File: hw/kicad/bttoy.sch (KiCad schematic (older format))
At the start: 4 parts

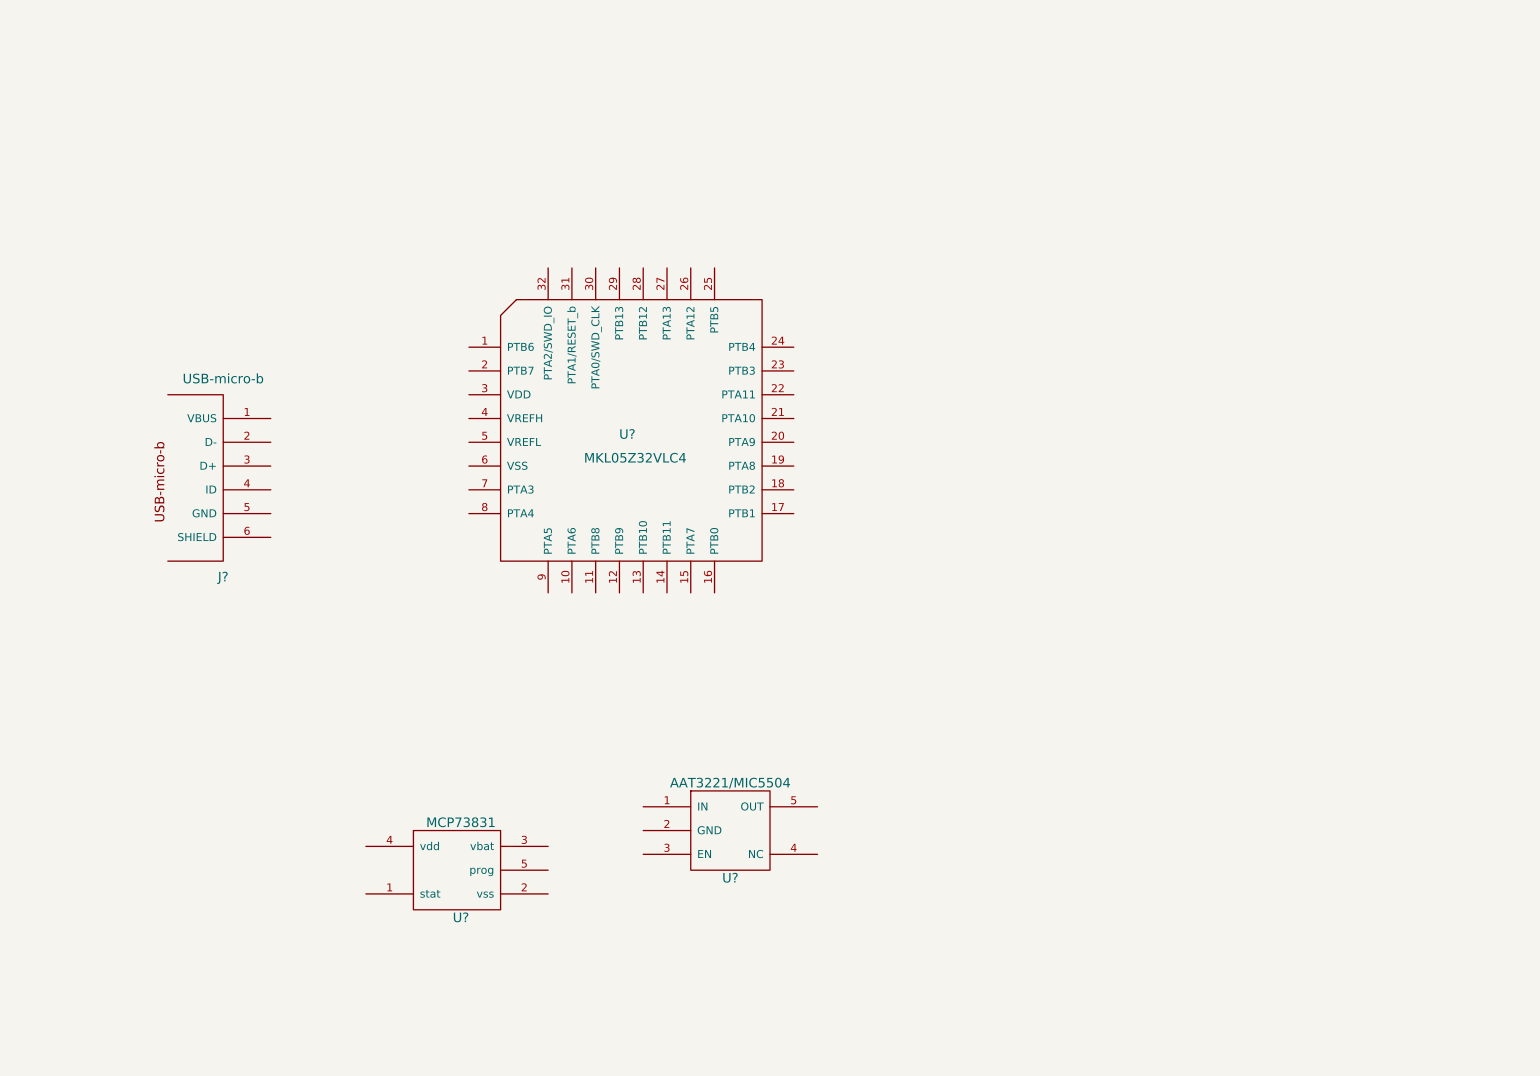
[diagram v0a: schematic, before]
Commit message: - start flushing out subsystems
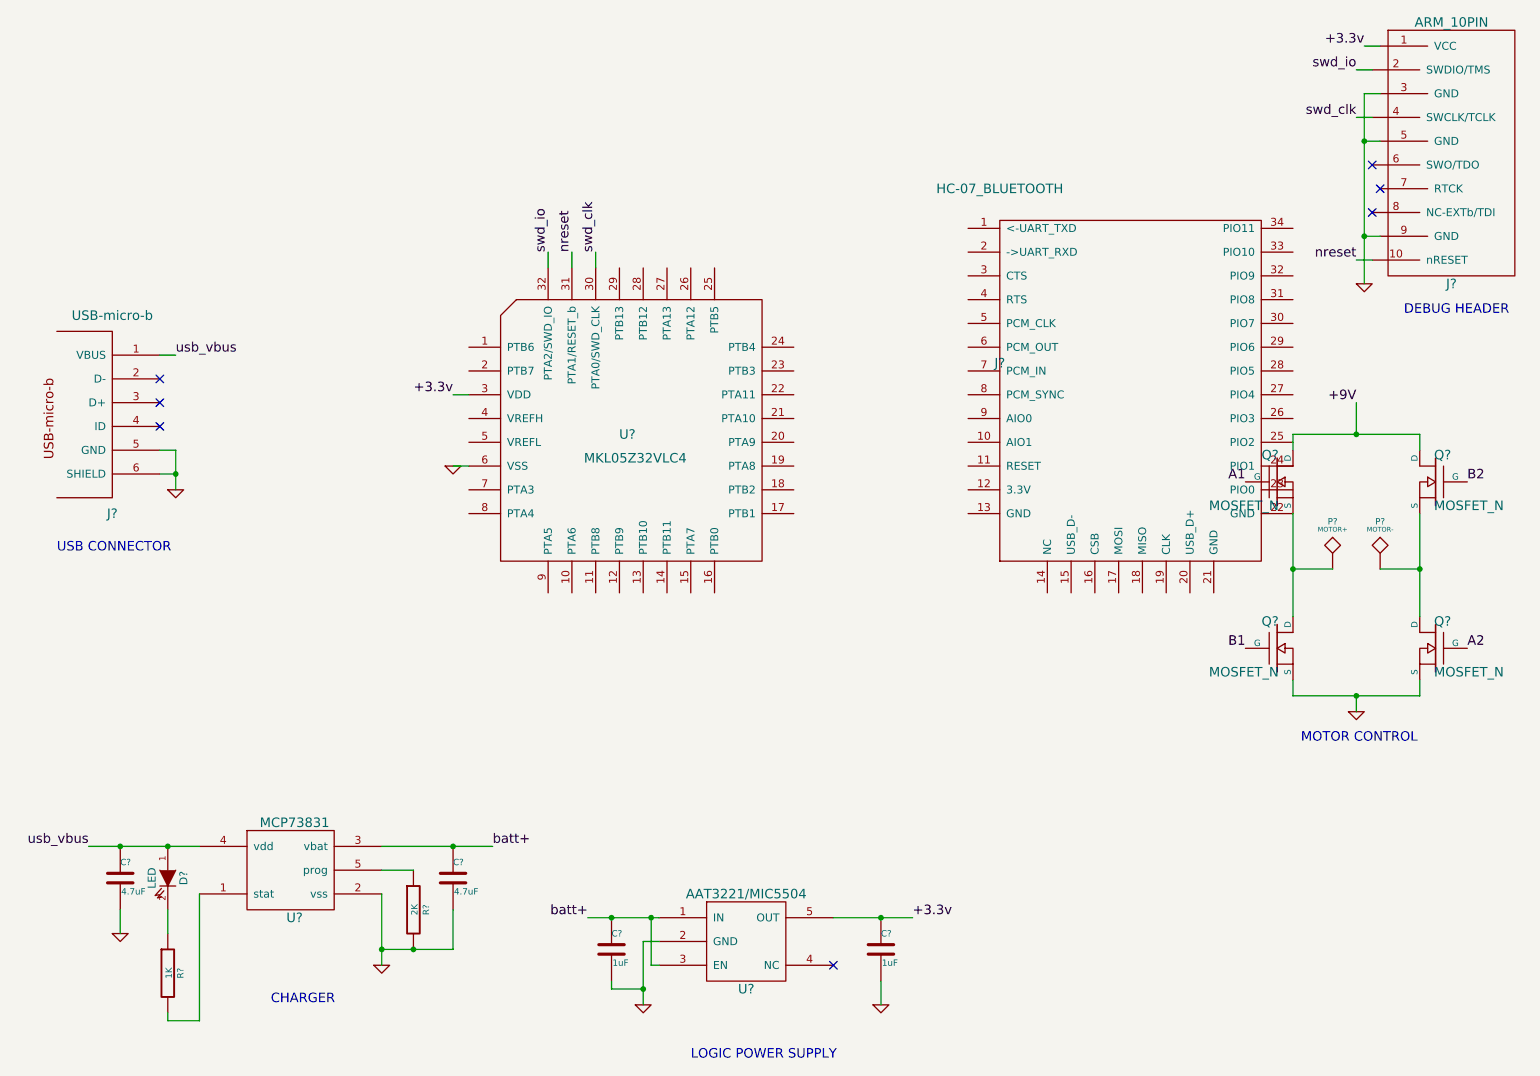
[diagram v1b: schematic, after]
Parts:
- added C? (x2): 4.7uF, symbol C
- added C? (x2): 1uF, symbol C
- added D?: LED, symbol LED
- added J?: ARM_10PIN, symbol ARM_10PIN
- added J?: HC-07_BLUETOOTH, symbol HC-07_BLUETOOTH
- added P?: MOTOR+, symbol TST
- added P?: MOTOR-, symbol TST
- added Q? (x4): MOSFET_N, symbol MOSFET_N
- added R?: 1K, symbol R
- added R?: 2K, symbol R
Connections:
- net +3.3v: now reaches U?.3 (VDD)
- net +3.3v: now also U?.5 (OUT), C?.1, J?.1 (VCC)
- net swd_clk: now reaches U?.30 (PTA0/SWD_CLK)
- net swd_clk: now also J?.4 (SWCLK/TCLK)
- net nreset: now reaches U?.31 (PTA1/RESET_b)
- net nreset: now also J?.10 (nRESET)
- net swd_io: now reaches U?.32 (PTA2/SWD_IO)
- net swd_io: now also J?.2 (SWDIO/TMS)
- net GND: now reaches U?.6 (VSS)
- net GND: now also J?.5 (GND), J?.6 (SHIELD), U?.2 (GND), U?.2 (vss), C?.2, C?.2, C?.2, C?.2, J?.3 (GND), J?.5 (GND), J?.9 (GND), Q?.S, Q?.S, R?.2
- net at U?.1 (stat): now also R?.2
- net batt+: now reaches U?.3 (vbat)
- net batt+: now also U?.1 (IN), U?.3 (EN), C?.1, C?.1
- net usb_vbus: now reaches U?.4 (vdd)
- net usb_vbus: now also J?.1 (VBUS), C?.1, D?.1 (A)
- net at U?.5 (prog): now also R?.1
- new net: J?.22 (GND), P?.1, Q?.D, Q?.S
- new net: P?.1, Q?.D, Q?.S
- new net: D?.2 (K), R?.1
- new net +9V: Q?.D, Q?.D
- new net A1: Q?.G
- new net A2: Q?.G
- new net B1: Q?.G
- new net B2: Q?.G
- no-connect marks 0 -> 7
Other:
- note added: "CHARGER"
- note added: "DEBUG HEADER"
- note added: "LOGIC POWER SUPPLY"
- note added: "MOTOR CONTROL"
- note added: "USB CONNECTOR"
- moved on the sheet: J?, U?
